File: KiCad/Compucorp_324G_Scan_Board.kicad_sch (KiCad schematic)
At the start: 31 parts, among them J1 Scan Interboard, J2 Power In, J4 From Keyboard, U1 BR 16252, U2 UHP480, U21 TMC1884 (TCL08), U3 UHP480, U4 TMC1869 (TCL02)

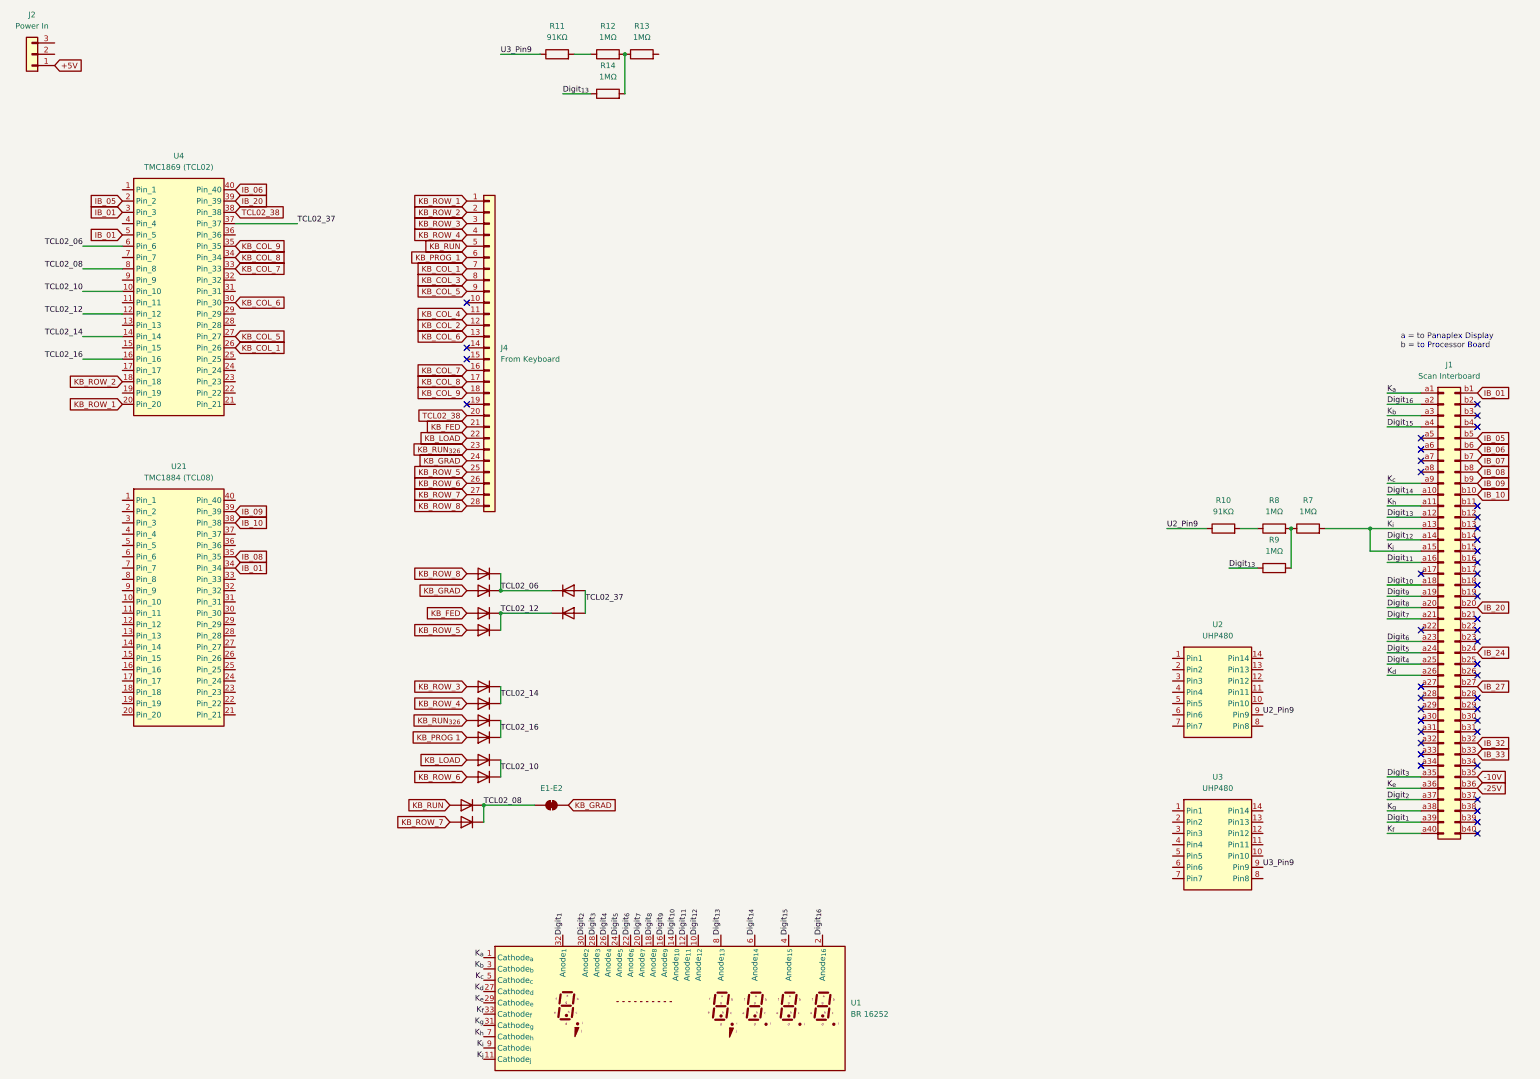
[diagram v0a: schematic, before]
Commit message: Update Compucorp_324G_Scan_Board.kicad_sch
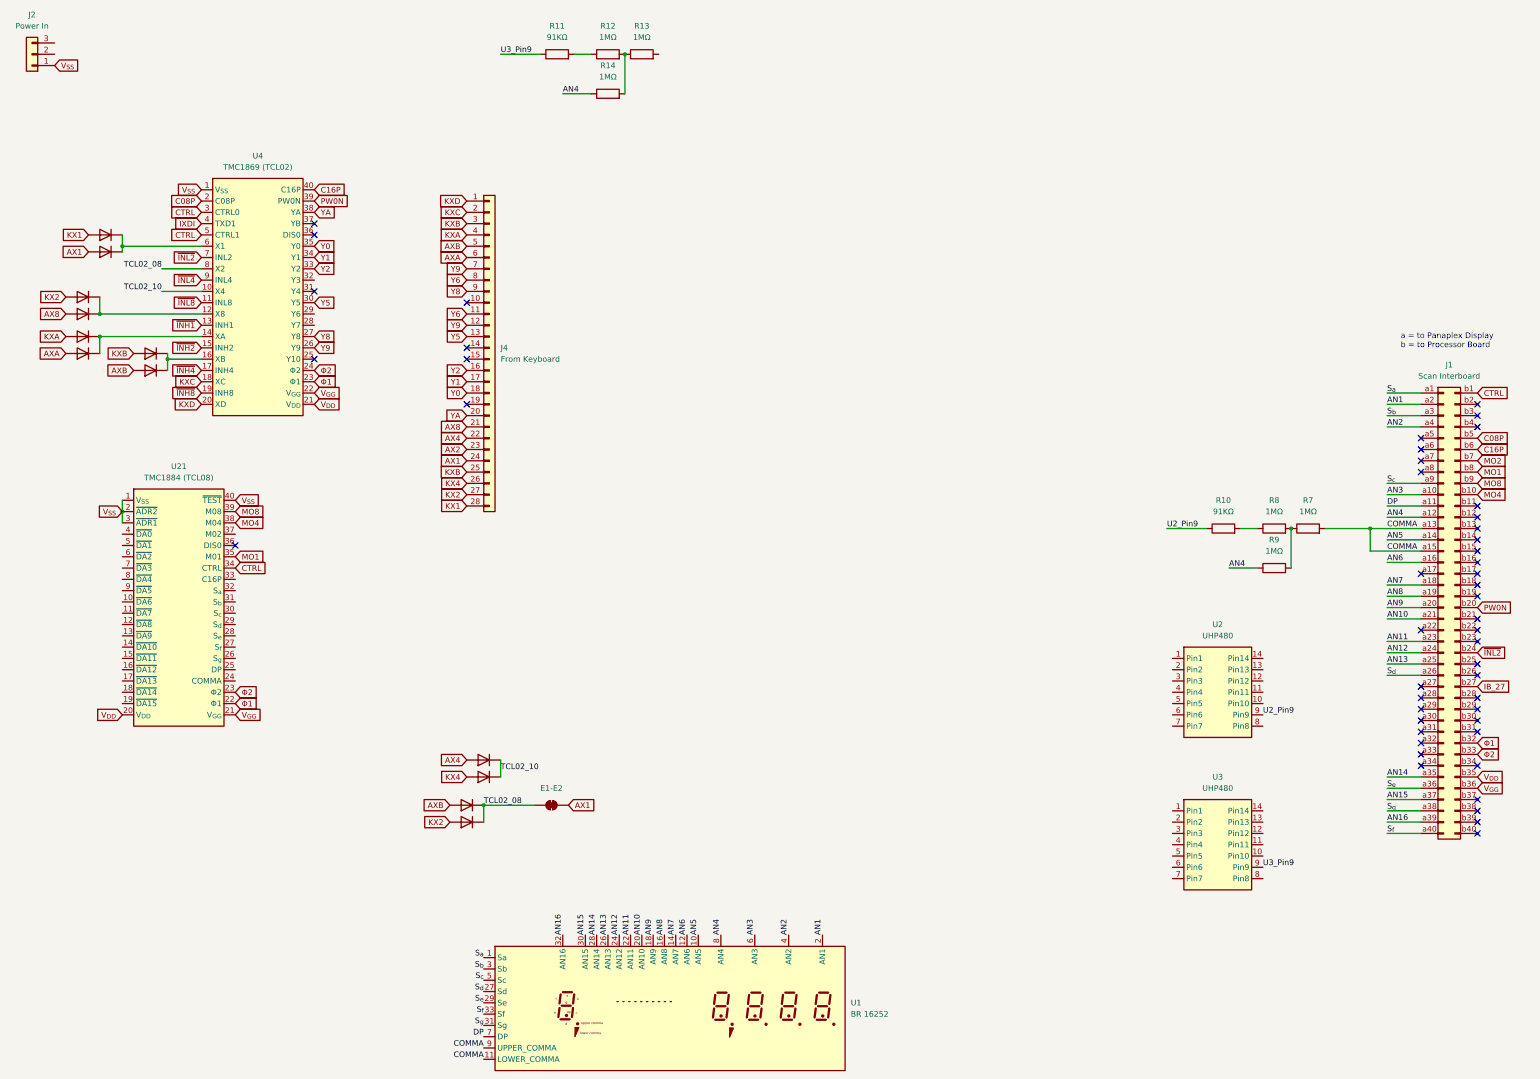
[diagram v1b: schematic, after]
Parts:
- removed D17, D18: D, symbol Device:D
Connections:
- net +5V is gone; now on net V_{SS}: J2.1 (Pin_1)
- net -10V is gone; now on net V_{DD}: J1.b35 (Pin_b35)
- net -25V is gone; now on net V_{GG}: J1.b36 (Pin_b36)
- net IB_24 is gone; now on net ~{INL2}: J1.b24 (Pin_b24)
- net IB_32 is gone; now on net Φ1: J1.b32 (Pin_b32)
- net IB_33 is gone; now on net Φ2: J1.b33 (Pin_b33)
- net KB_COL_2 is gone; now on net Y9: J4.12 (Pin_12)
- net KB_COL_4 is gone; now on net Y6: J4.11 (Pin_11)
- net KB_ROW_7 is gone; now on net KX2: D7.2 (A), J4.27 (Pin_27)
- net KB_RUN is gone; now on net AXB: D6.2 (A), J4.5 (Pin_5)
- net V_{SS}: now reaches U21.1 (V_{SS})
- net V_{SS}: now also U21.2 (~{ADR2}), U21.3 (~{ADR1}), U21.40 (~{TEST}), U4.1 (V_{SS})
- net V_{DD}: now reaches U21.20 (V_{DD})
- net V_{DD}: now also U4.21 (V_{DD})
- net V_{GG}: now reaches U21.21 (V_{GG})
- net V_{GG}: now also U4.22 (V_{GG})
- net Φ1: now reaches U21.22 (Φ1)
- net Φ1: now also U4.23 (Φ1)
- net Φ2: now reaches U21.23 (Φ2)
- net Φ2: now also U4.24 (Φ2)
- net ~{INL8}: now reaches U4.11 (INL8)
- net ~{INH1}: now reaches U4.13 (INH1)
- net ~{INH2}: now reaches U4.15 (INH2)
- net ~{INH4}: now reaches U4.17 (INH4)
- net ~{INH8}: now reaches U4.19 (INH8)
- net IXDI: now reaches U4.4 (TXD1)
- net ~{INL2}: now reaches U4.7 (INL2)
- net ~{INL4}: now reaches U4.9 (INL4)
- net Digit_{10} renamed AN7
- net Digit_{11} renamed AN6
- net Digit_{12} renamed AN5
- net Digit_{13} renamed AN4
- net Digit_{14} renamed AN3
- net Digit_{15} renamed AN2
- net Digit_{16} renamed AN1
- net Digit_{1} renamed AN16
- net Digit_{2} renamed AN15
- net Digit_{3} renamed AN14
- net Digit_{4} renamed AN13
- net Digit_{5} renamed AN12
- net Digit_{6} renamed AN11
- net Digit_{7} renamed AN10
- net Digit_{8} renamed AN9
- net Digit_{9} renamed AN8
- net IB_01 renamed CTRL
- net IB_05 renamed C08P
- net IB_06 renamed C16P
- net IB_07 renamed MO2
- net IB_08 renamed MO1
- net IB_09 renamed MO8
- net IB_10 renamed MO4
- net IB_20 renamed PW0N
- net KB_COL_1 renamed Y9
- net KB_COL_3 renamed Y6
- net KB_COL_5 renamed Y8
- net KB_COL_6 renamed Y5
- net KB_COL_7 renamed Y2
- net KB_COL_8 renamed Y1
- net KB_COL_9 renamed Y0
- net KB_FED renamed AX8
- net AX8: now also D16.2 (A); no longer D1.2 (A)
- net KB_GRAD renamed AX1
- net KB_LOAD renamed AX4
- net KB_PROG 1 renamed AXB
- net KB_PROG_1 renamed AXA
- net AXA: now also D2.2 (A)
- net KB_ROW_1 renamed KXD
- net KB_ROW_2 renamed KXC
- net KB_ROW_3 renamed KX2
- net KX2: no longer J4.3 (Pin_3)
- net KB_ROW_4 renamed KXA
- net KXA: now also D1.2 (A); no longer D16.2 (A)
- net KB_ROW_5 renamed KXB
- net KXB: now also D13.2 (A), J4.3 (Pin_3); no longer D2.2 (A)
- net KB_ROW_6 renamed KX4
- net KB_ROW_8 renamed KX1
- net KB_RUN_{326} renamed AX2
- net AX2: no longer D13.2 (A)
- net K_{a} renamed S_{a}
- net K_{b} renamed S_{b}
- net K_{c} renamed S_{c}
- net K_{d} renamed S_{d}
- net K_{e} renamed S_{e}
- net K_{f} renamed S_{f}
- net K_{g} renamed S_{g}
- net K_{h} renamed DP
- net K_{i} renamed COMMA
- net TCL02_06: no longer names the net of D5.1 (K), D8.1 (K), U4.6 (X1)
- net TCL02_12: no longer names the net of D1.1 (K), D2.1 (K)
- net TCL02_12: now also U4.14 (XA); no longer U4.12 (Pin_12)
- net TCL02_14: no longer names the net of D14.1 (K), D16.1 (K)
- net TCL02_14: now also U4.12 (X8); no longer U4.14 (Pin_14)
- net TCL02_16: no longer names the net of D13.1 (K), D15.1 (K), U4.16 (XB)
- net TCL02_37: no longer names the net of U4.37 (YB)
- net TCL02_38 renamed YA
- no-connect marks 44 -> 49
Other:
- moved on the sheet: U4
